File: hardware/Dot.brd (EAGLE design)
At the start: 23.3 x 31.5 mm, 25 parts, among them IC1 CAT24M010TS, U1 ATMEGA328P-MU-QFN32, U2 TMP102

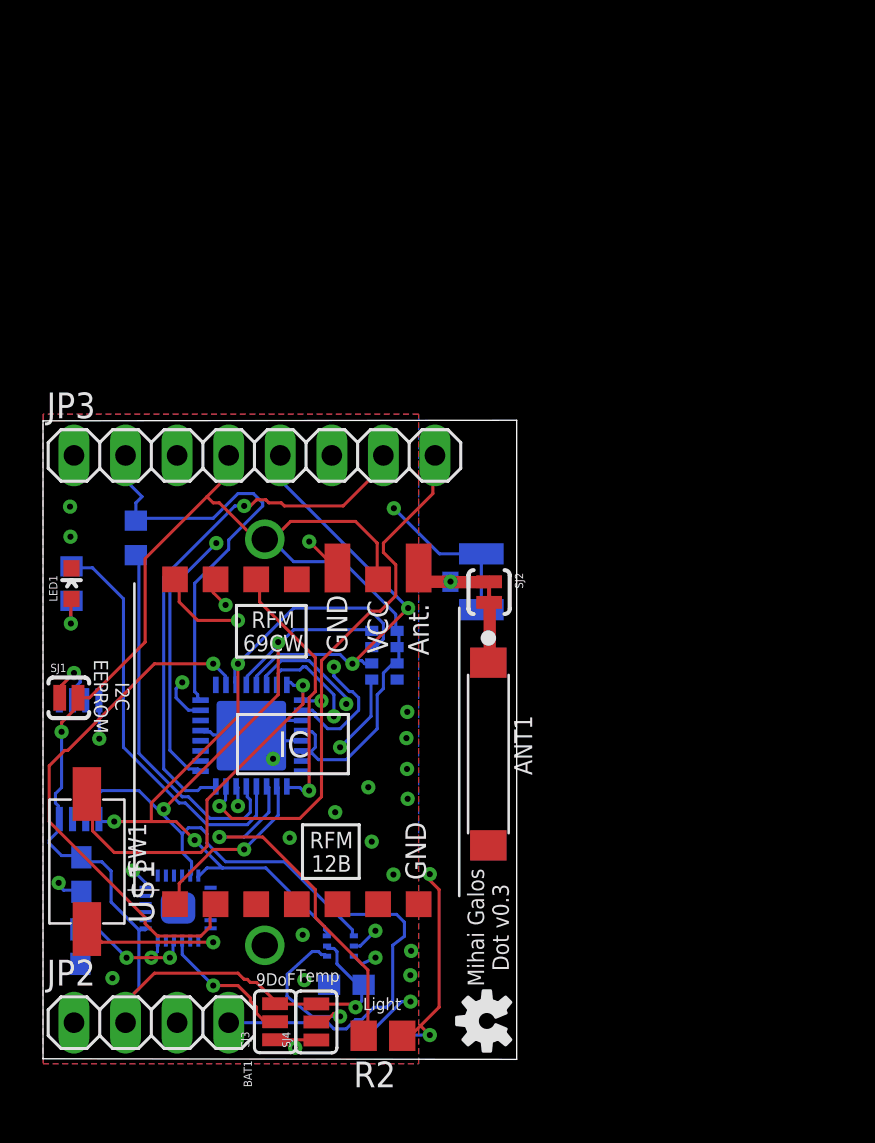
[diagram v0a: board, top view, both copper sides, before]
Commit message: v0.5
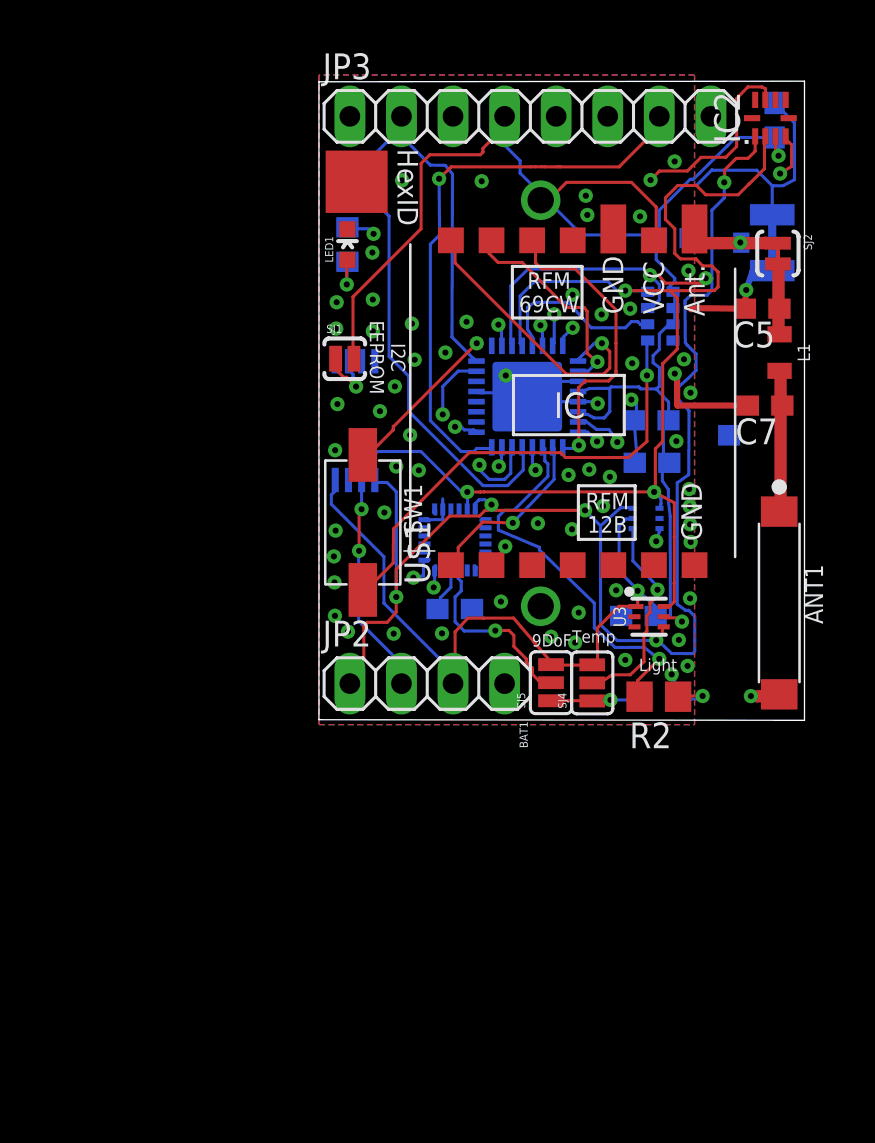
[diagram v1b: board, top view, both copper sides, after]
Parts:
- removed SJ3: (no value), SparkFun:SJ_3
- removed U$3: MPU-9250, invensense:LEAD-QFN24
- added C4, C8: 0.1uF, resistor:C0603
- added C5, C7: (no value), resistor:C0603
- added C6: 1uF, resistor:C0603
- added IC2: SI1145, silabs:QFN-10
- added L1: 3.3µH/±20%/450mA, SparkFun-Coils:0805
- added SJ5: (no value), SparkFun:SJ_3
- added U3: ISL29125, SparkFun-Sensors:ODFN-6
- added U4: 9DoF IMU, SparkFun-Sensors:QFN24-3X3
- R3: value 1kΩ -> 10kΩ
- moved C1 42.8 mm to (31.0, 40.2), turned to 180 degrees
- moved C2 36.9 mm to (30.0, 29.1), turned to 0 degrees
- moved C3 31.6 mm to (30.0, 31.2)
- moved LOGO1 27.4 mm to (35.7, 25.2), flipped to the bottom
- moved U2 25.9 mm to (29.7, 26.4)
- moved X1 22.0 mm to (35.9, 39.9)
- moved SJ2 21.9 mm to (36.2, 39.4)
- moved IC1 21.5 mm to (16.6, 31.2)
- moved JP3 21.5 mm to (24.0, 46.2)
- moved LED1 21.5 mm to (15.0, 39.9)
- moved R1 21.5 mm to (15.0, 39.9)
- moved R3 21.5 mm to (30.4, 17.5)
- moved R7 21.5 mm to (30.4, 36.3)
- moved SJ4 21.5 mm to (27.1, 18.3)
- moved U$1 21.5 mm to (26.1, 31.6)
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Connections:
- removed net ANT_2: ANT1.1, SJ2.2
- removed net N$8: C2.1, U$3.10
- new net ANT: ANT1.1, C5.1, L1.1, SJ2.2
- new net INT_RGB: U1.7, U3.5
- new net INT_UV: IC2.4, U1.8
- new net N$11: C8.1, U4.10
- new net N$14: SJ5.2, U4.9
- net +3V3: now also C2.1, C4.1, C6.1, IC2.3, JP2.3, SJ5.3, U3.1, U4.13; no longer JP2.2, SJ3.3, U$3.13
- net GND: now also C4.2, C5.2, C6.2, C7.2, C8.2, IC2.8, JP2.4, SJ5.1, U3.3, U4.18, U4.20; no longer JP2.1, SJ3.1, U$3.18
- net MOVE_INT: now also U4.12; no longer U$3.12
- net N$9: now also C7.1, L1.2; no longer SJ3.2, U$3.9
- net SCL: now also IC2.2, JP2.2, U3.6, U4.23; no longer JP2.4, U$3.23
- net SDA: now also IC2.1, JP2.1, U3.4, U4.24; no longer JP2.3, U$3.24
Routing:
- net SDA: track 45.5 -> 84.6 mm, vias 3 -> 7
- net +3V3: track 86.7 -> 119.4 mm, vias 2 -> 3
- net INT_UV: track 0.00 -> 26.1 mm, vias 0 -> 2
- net SCL: track 54.9 -> 74.1 mm, vias 2 -> 5
- net INT_RGB: track 0.00 -> 13.8 mm, vias 0 -> 2
- net RIRQ: track 26.1 -> 14.5 mm, vias 1 -> 2
- net N$14: track 0.00 -> 9.39 mm, vias 0 -> 1
- net GND: track 48.7 -> 57.0 mm, vias 25 -> 63
- net TXD: track 23.9 -> 15.8 mm
- net N$9: track 6.97 -> 0.00 mm, vias 1 -> 0
- net N$12: track 0.00 -> 6.95 mm
- net SCK: track 21.4 -> 26.3 mm
- net PUSH: track 19.0 -> 14.2 mm, vias 1 -> 2
- net ANT_1: track 3.94 -> 0.00 mm
- net RSCK: track 14.6 -> 10.6 mm, vias 2 -> 1
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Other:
- board size 23.3 x 31.5 mm -> 23.9 x 31.5 mm
- board text added: "Dot v0.5"
- board text added: "HexID"
- board text removed: "01.2017"
- board text removed: "Mihai Galos Dot v0.3"

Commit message: v1.3
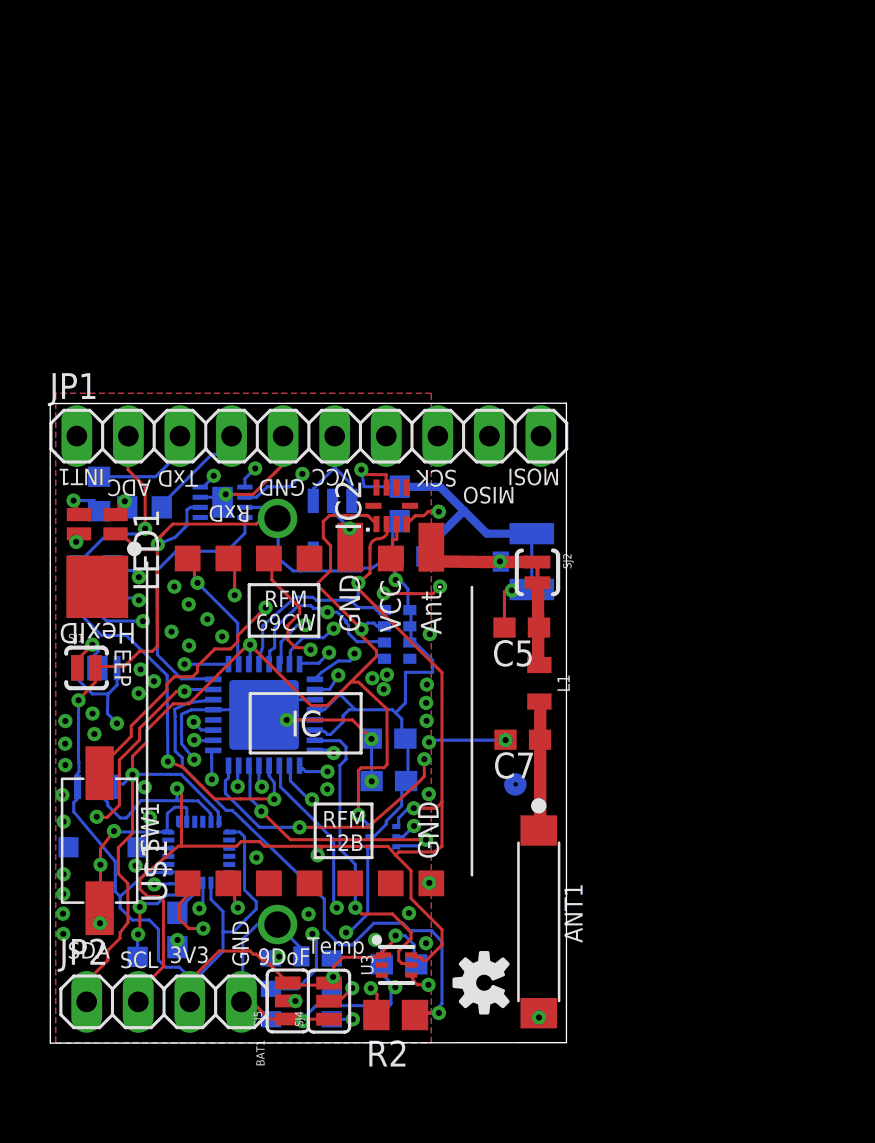
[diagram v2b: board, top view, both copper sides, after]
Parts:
- removed JP3: (no value), pinhead:1X08
- removed R1: 150Ω, resistor:R0603
- added JP1: (no value), pinhead:1X10
- added R5: 130Ω, resistor:R0603
- added R6, R8: 30Ω, resistor:R0603
- added SPK1: SMT-0540-S-R, adafruit:SMT-0540-S-R
- added U$3: AT45DB641E, AT45DB641E:UDFN-8
- added U$4: LDCL015, LDCL015:SOT23-5
- added U5: BMP18, Seeed-OPL-sensor:LGA7-1.5-3.8X3.6MM
- LED1: value (none) -> GM1WA55311A; device SparkFun:LED-0603 -> led:GM1WA55311A
- moved IC2 26.7 mm to (17.2, 27.0)
- moved C6 26.4 mm to (17.6, 27.1)
- moved LOGO1 25.9 mm to (21.7, 3.49), flipped to the top
- moved R4 22.9 mm to (2.58, 24.0)
- moved U3 21.2 mm to (17.4, 4.37)
- moved C8 20.9 mm to (6.62, 6.09), turned to 270 degrees
- moved C4 20.8 mm to (17.5, 4.39)
- moved C2 20.3 mm to (17.0, 13.4)
- moved R3 20.3 mm to (17.4, 1.83)
- moved R7 20.3 mm to (17.4, 20.6)
- moved C1 20.3 mm to (18.1, 24.5)
- moved C3 20.3 mm to (17.0, 15.5)
- moved JP2 20.3 mm to (5.96, 2.55)
- moved SJ4 20.3 mm to (14.1, 2.58)
- moved SJ5 20.3 mm to (12.1, 2.59)
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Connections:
- removed net ADC1: JP3.2, R4.1, U1.24
- removed net N$7: LED1.A, R1.2
- new net ADC: JP1.2, R4.1, U1.19
- new net BUZZER: SPK1.+, U1.23
- new net FLASH_CS: U$3.4, U1.24
- new net N$1: LED1.3, R8.1
- new net N$15: LED1.1, R5.1
- new net RXD: JP1.4, R5.2, U1.30
- new net VIN: JP1.6, U$4.1, U$4.3
- net +3V3: now also LED1.4, U$3.3, U$3.6, U$4.5, U1.18, U4.1, U4.8, U5.2, U5.3; no longer JP3.4
- net GND: now also JP1.5, SPK1.-, SW1.2, U$3.7, U$3.THERM, U$4.2, U4.11, U5.7; no longer JP3.3, LED1.C, R7.8
- net LED: now also R8.2; no longer R1.1
- net LIGHT_SENSE: now also U1.22; no longer U1.23
- net MISO: now also JP1.9, U$3.8; no longer JP3.7
- net MOSI: now also JP1.10, U$3.1; no longer JP3.8
- net MOVE_INT: now also U1.25; no longer U1.30
- net N$4: now also LED1.2, R6.1; no longer R7.1, SW1.2
- net PUSH: now also JP1.1, U1.1; no longer U1.32
- net RIRQ: now also U1.32; no longer U1.26
- net RSEL: now also U1.26; no longer U1.1
- net RST: now also JP1.7; no longer JP3.5
- net SCK: now also JP1.8, U$3.2; no longer JP3.6
- net SCL: now also U5.5
- net SDA: now also U5.6
- net TXD: now also JP1.3, R6.2; no longer JP3.1
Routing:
- net GND: track 57.0 -> 134.5 mm, vias 63 -> 57
- net MOSI: track 23.0 -> 49.7 mm, vias 1 -> 2
- net ADC: track 0.00 -> 21.3 mm, vias 0 -> 3
- net N$4: track 23.2 -> 2.39 mm
- net MISO: track 28.2 -> 48.9 mm, vias 1 -> 5
- net PUSH: track 14.2 -> 34.0 mm
- net RXD: track 0.00 -> 19.1 mm, vias 0 -> 1
- net ADC1: track 18.2 -> 0.00 mm
- net SCK: track 26.3 -> 41.4 mm, vias 1 -> 2
- net BUZZER: track 0.00 -> 14.8 mm, vias 0 -> 3
- net FLASH_CS: track 0.00 -> 13.3 mm
- net +3V3: track 119.4 -> 128.9 mm, vias 3 -> 7
- net INT_UV: track 26.1 -> 17.1 mm
- net SCL: track 74.1 -> 82.7 mm
- net RSEL: track 14.2 -> 6.23 mm
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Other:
- board size 23.9 x 31.5 mm -> 25.4 x 31.5 mm
- board text added: "05.2017"
- board text added: "3V3"
- board text added: "ADC"
- board text added: "Dot v1.3"
- board text added: "EEP"
- board text added: "GND"
- board text added: "INT1"
- board text added: "MISO"
- board text added: "MOSI"
- board text added: "Mihai Galos"
- board text added: "RxD"
- board text added: "SCK"
- board text added: "SCL"
- board text added: "SDA"
- board text added: "TxD"
- board text added: "VCC"
- board text removed: "Dot v0.5"
- board text removed: "I2C EEPROM"
- board text removed: "Light"
